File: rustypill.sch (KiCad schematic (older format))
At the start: 53 parts, among them J1 USB, J2 PROG, J3 GPIOB, J4 GPIOA, J5 HD44780, J6 IDC_10P, J7 I2C, J8 Micro_SD_Card, Q1 S8050, SW1 Reset, U1 AMS1117-3.3, U2 AT24C512C-SSHD-T, U3 ESP-12F, U4 STM32F411CEUx, U5 PCF8574, U6 DS3231, Y1 8MHz

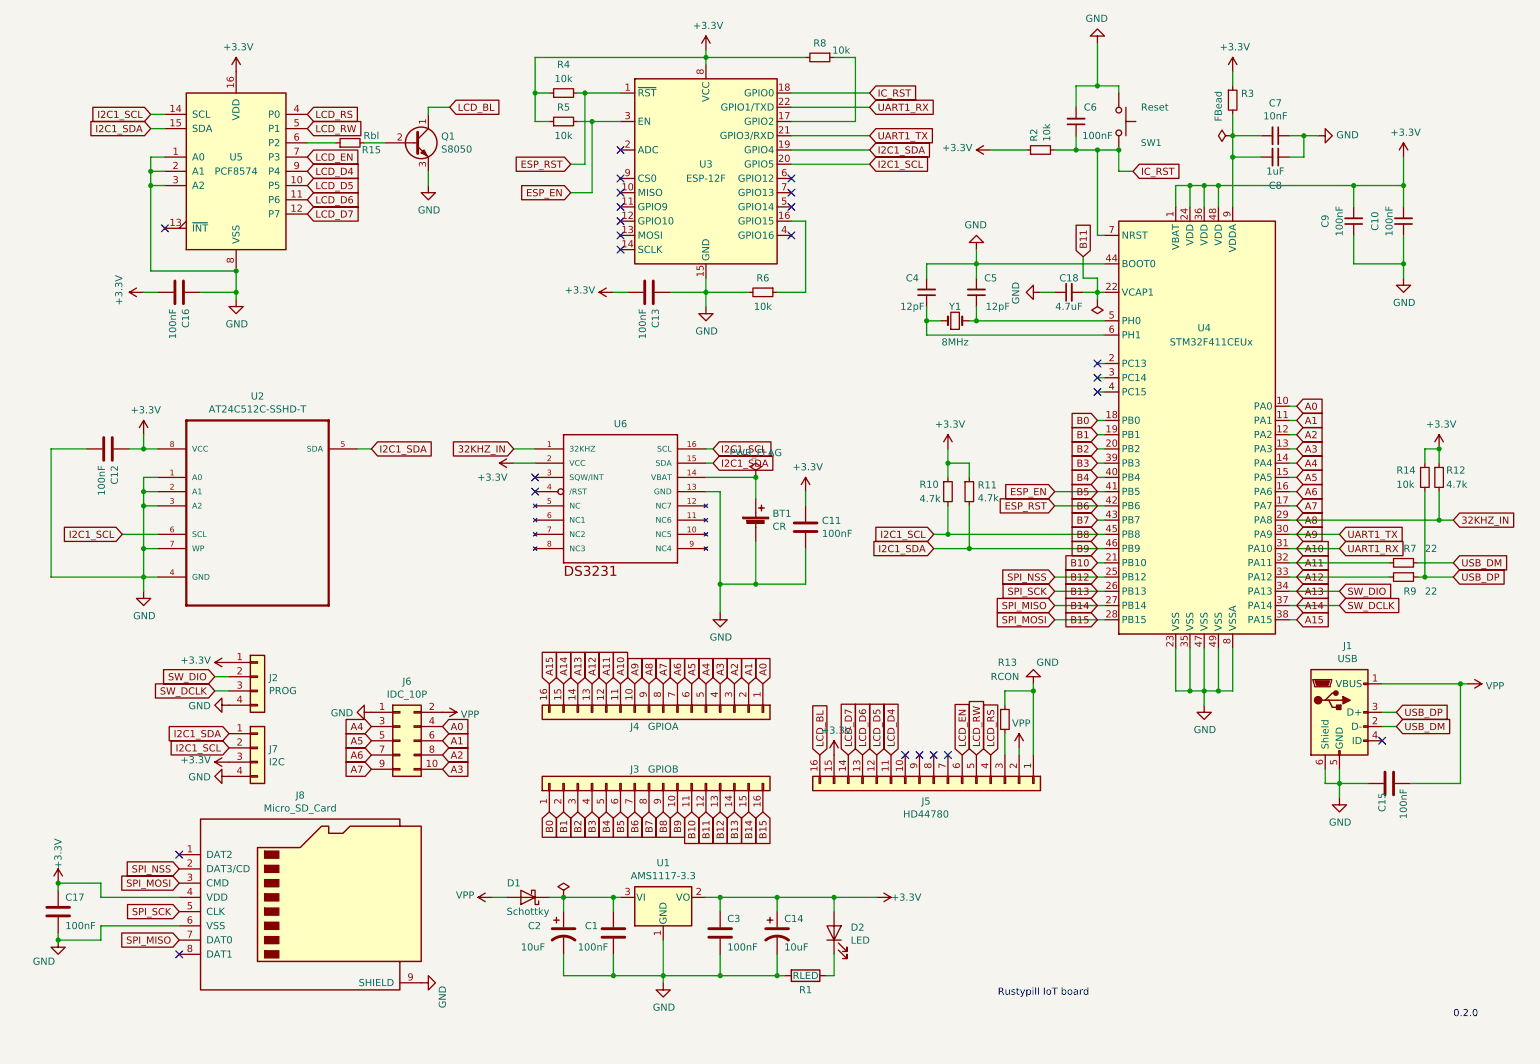
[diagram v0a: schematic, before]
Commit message: ...
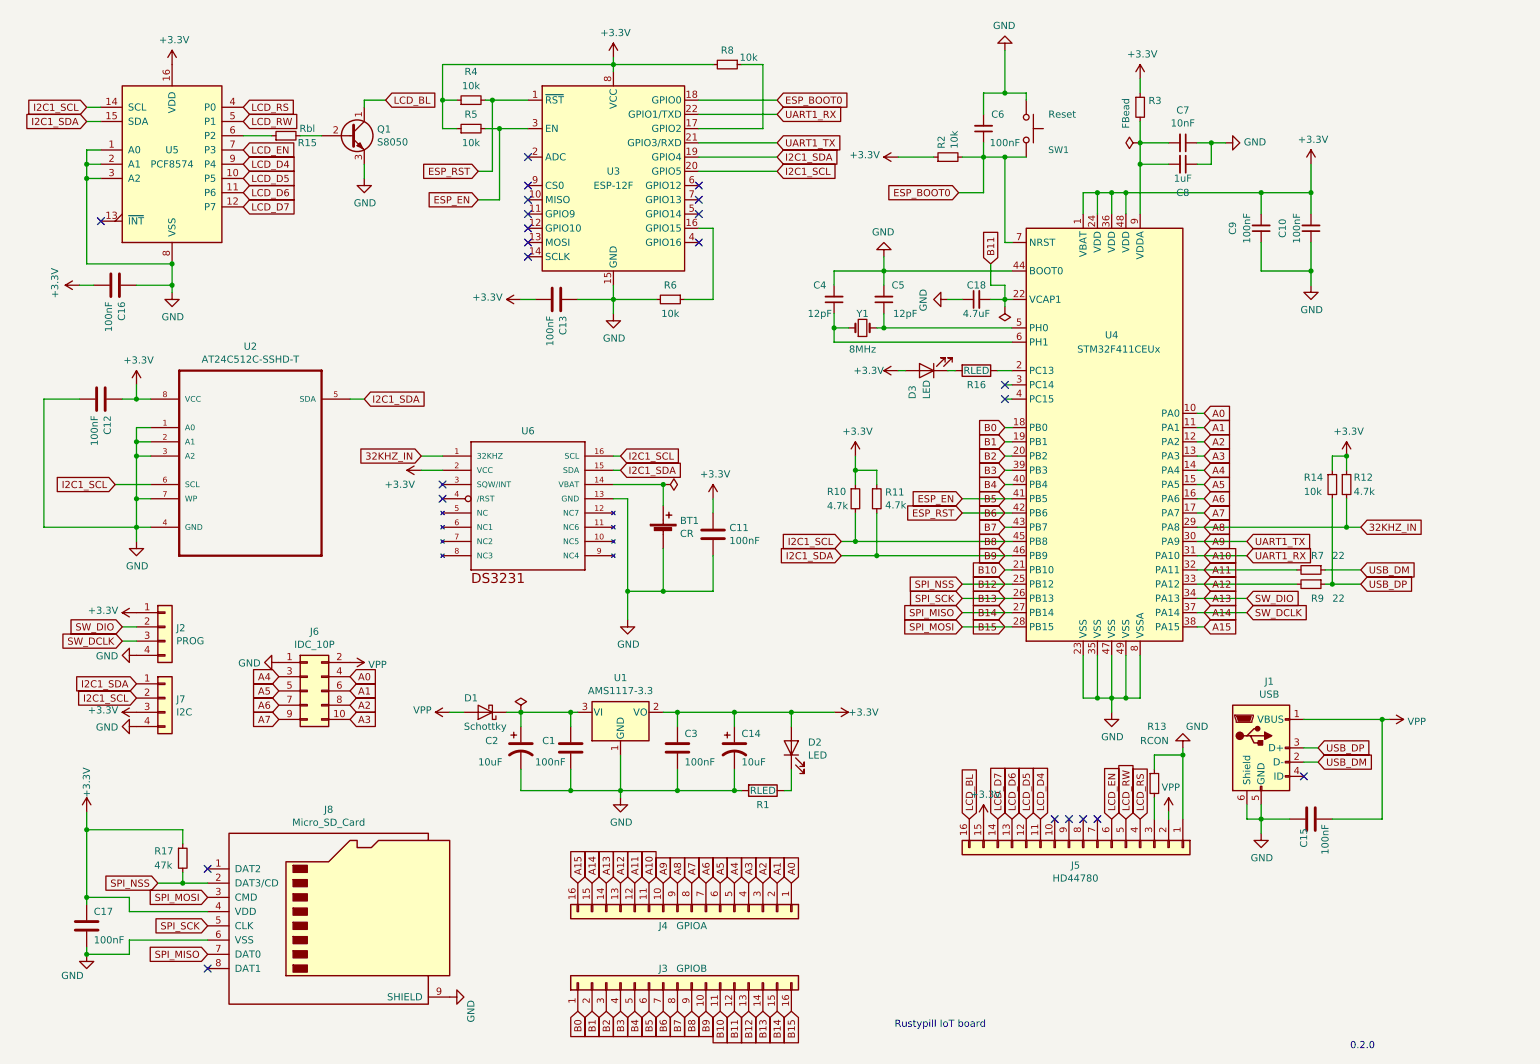
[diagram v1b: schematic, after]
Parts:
- added D3: LED, LEDs:LED_0805_HandSoldering, symbol Device:LED
- added R16: RLED, Resistors_SMD:R_0805_HandSoldering, symbol Device:R
- added R17: 47k, Resistors_SMD:R_0805_HandSoldering, symbol Device:R_Small
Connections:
- net +3V3: now also D3.2 (A), R17.1
- net B12: now also R17.2
- net at U4.2 (PC13): now also R16.1
- net IC_RST renamed ESP_BOOT0
- new net: D3.1 (K), R16.2
- no-connect marks 24 -> 23
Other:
- moved on the sheet: BT1, C1, C10, C11, C12, C13, C14, C15, C16, C17, C18, C2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
